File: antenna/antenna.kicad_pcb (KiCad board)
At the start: 2 copper layers, 50 x 43.3 mm, 17 parts, among them J1 Conn_01x05_Pin, J2 Conn_01x05_Pin, J3 Conn_01x05_Pin, J5 USB_C_Receptacle, U1 ESP32-C3-WROOM-02, U2 AMS1117-3.3

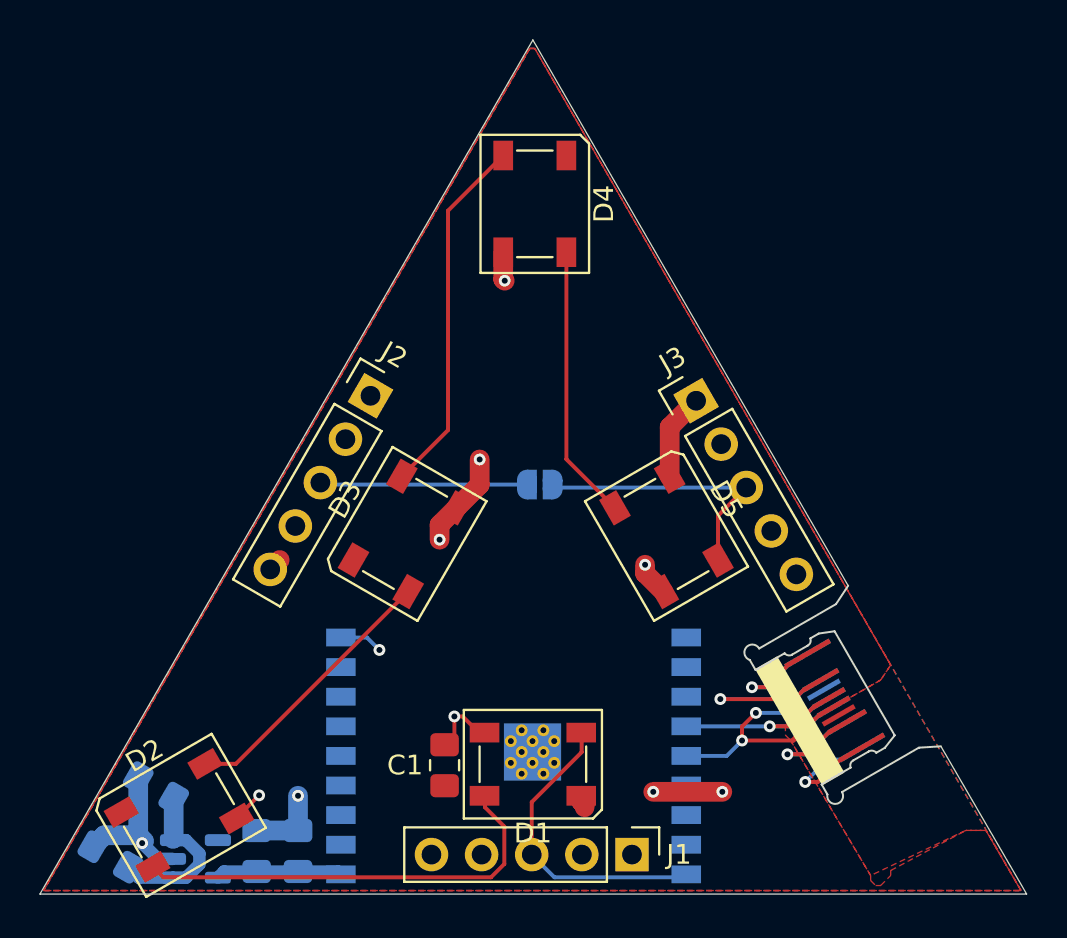
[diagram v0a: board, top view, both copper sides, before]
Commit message: great success!
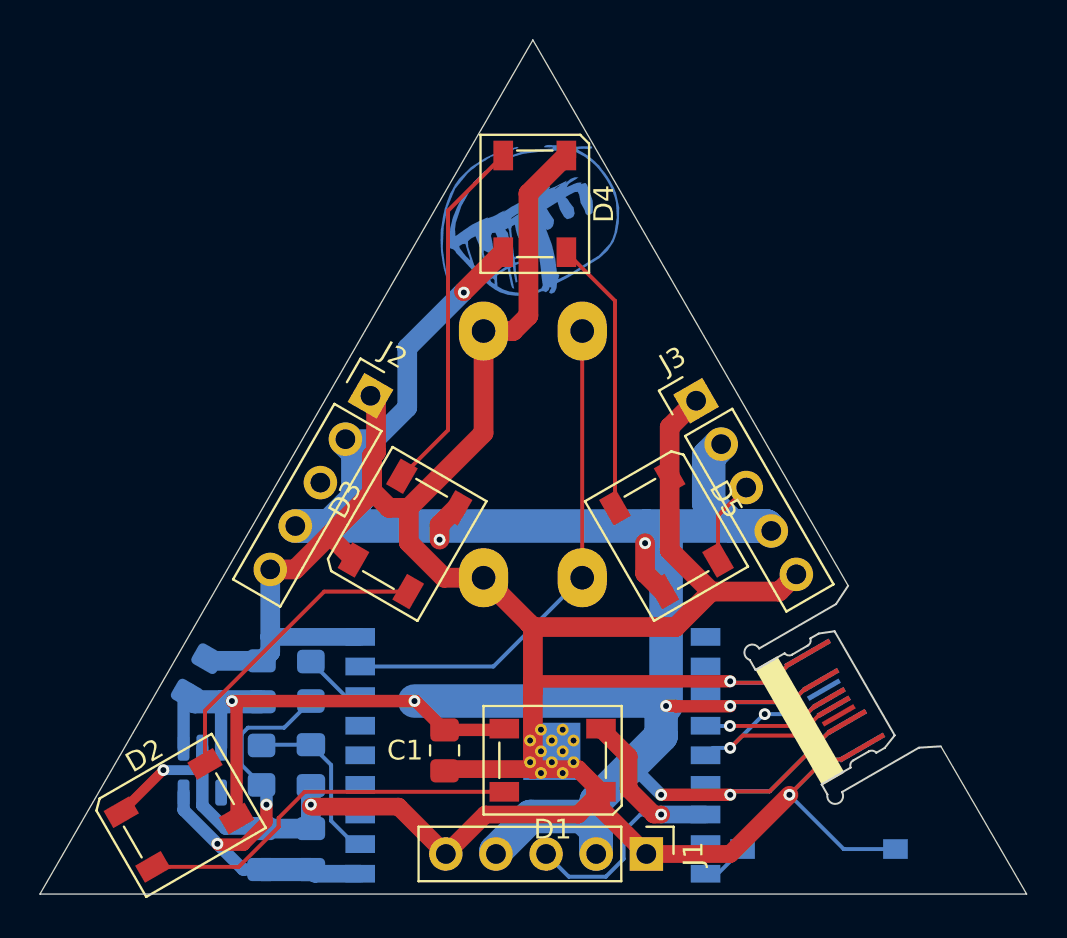
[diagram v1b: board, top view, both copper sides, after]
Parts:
- removed JP1: SolderJumper_2_Open, Jumper:SolderJumper-2_P1.3mm_Open_RoundedPad1.0x1.5mm
- added C6: 4u7F, Capacitor_SMD:C_0805_2012Metric_Pad1.18x1.45mm_HandSolder, B.Cu at (138.8, 86.8)
- added R1: 10k, Resistor_SMD:R_0805_2012Metric_Pad1.20x1.40mm_HandSolder, B.Cu at (136.2, 86.8)
- added R2: 10k, Resistor_SMD:R_0805_2012Metric_Pad1.20x1.40mm_HandSolder, B.Cu at (138.8, 82.5)
- added SW1: SW_Push, 0_NRD_footprints:SW_PUSH-12mm_Wuerth-430456085736, B.Cu at (147.5, 64.8)
- added SW2: SW_Push, Button_Switch_SMD:SW_Tactile_SPST_NO_Straight_CK_PTS636Sx25SMTRLFS, B.Cu at (164.5, 91.0)
- C1: value C -> 4u7F
- C2: value 100nF -> 4u7F
- moved C4 10.2 mm to (133.0, 82.2), turned to 60 degrees
- moved C5 7.60 mm to (136.2, 82.5), turned to 90 degrees
- moved U2 4.51 mm to (133.2, 87.0), turned to -90 degrees
- moved C3 2.75 mm to (138.8, 91.0)
- moved C2 1.85 mm to (136.2, 91.0)
- moved D1 1.02 mm to (151.0, 86.5)
- moved U1 0.98 mm to (150.0, 86.2)
- moved C1 0.75 mm to (145.5, 86.0)
- moved J1 0.73 mm to (155.8, 91.2)
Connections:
- J2 pad 3: Net-(J2-Pin_3) -> unconnected-(J2-Pin_3-Pad3)
- U1 pad 16: unconnected-(U1-IO2-Pad16) -> Net-(D1-DIN)
- U1 pad 18: Net-(D1-DIN) -> Net-(U1-IO0)
- U1 pad 2: unconnected-(U1-EN-Pad2) -> Net-(U1-EN)
- U1 pad 7: unconnected-(U1-IO8-Pad7) -> Net-(U1-IO8)
- U1 pad 8: unconnected-(U1-IO9-Pad8) -> Net-(U1-IO9)
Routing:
- net GND: track 28.2 -> 178.2 mm, vias 5 -> 4
- net +5V: track 39.1 -> 154.0 mm, vias 10 -> 9
- net Net-(U1-IO9): track 0.00 -> 25.6 mm
- net Net-(U1-3V3): track 6.43 -> 23.3 mm, vias 0 -> 2
- net Net-(J2-Pin_3): track 10.5 -> 0.00 mm
- net Net-(D5-DOUT): track 14.1 -> 4.26 mm
- net Net-(U1-EN): track 0.00 -> 8.76 mm
- net /D-: track 9.54 -> 5.89 mm
- net Net-(U1-IO8): track 0.00 -> 3.22 mm
- net Net-(D1-DOUT): track 22.2 -> 19.7 mm
- net Net-(U1-IO0): track 0.00 -> 2.39 mm
- net Net-(D2-DOUT): track 13.9 -> 15.5 mm
- net Net-(D1-DIN): track 15.6 -> 16.5 mm, vias 0 -> 1
- net /D+: track 12.3 -> 11.6 mm
- removed copper zone on B.Cu, net +5V
- removed copper zone on F.Cu, net +5V
- removed copper zone on F.Cu, net GND
